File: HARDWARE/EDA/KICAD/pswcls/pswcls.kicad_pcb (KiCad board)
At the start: 2 copper layers, 60.9 x 27 mm, 22 parts, among them J1 PW_RELAY, J2 PW_LOGIC_RELAY, J3 RELAY_TERMINAL, J4 NC_Relay, J5 NA_Relay, J6 C_Relay, K1 G5LE-1, Q1 BC549, U1 4N35

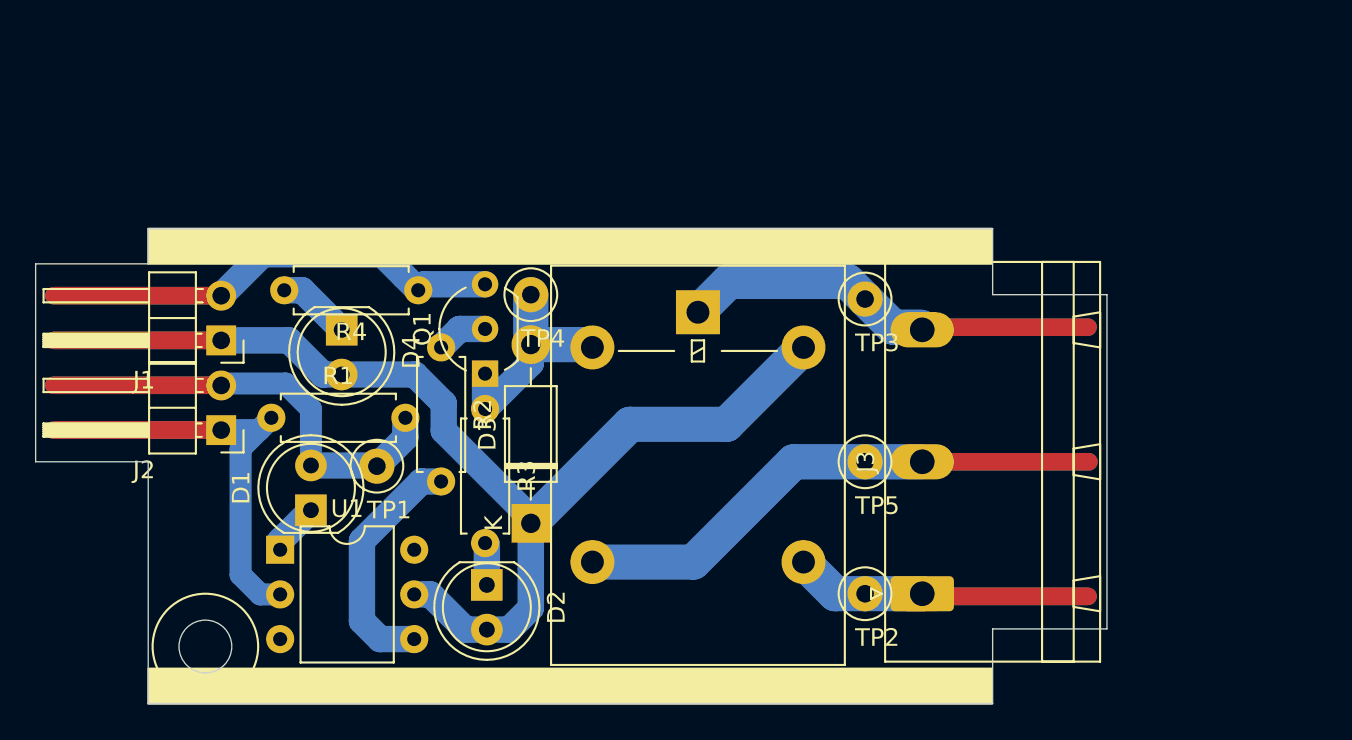
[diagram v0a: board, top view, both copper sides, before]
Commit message: pre adjust pcb and adjust schematic
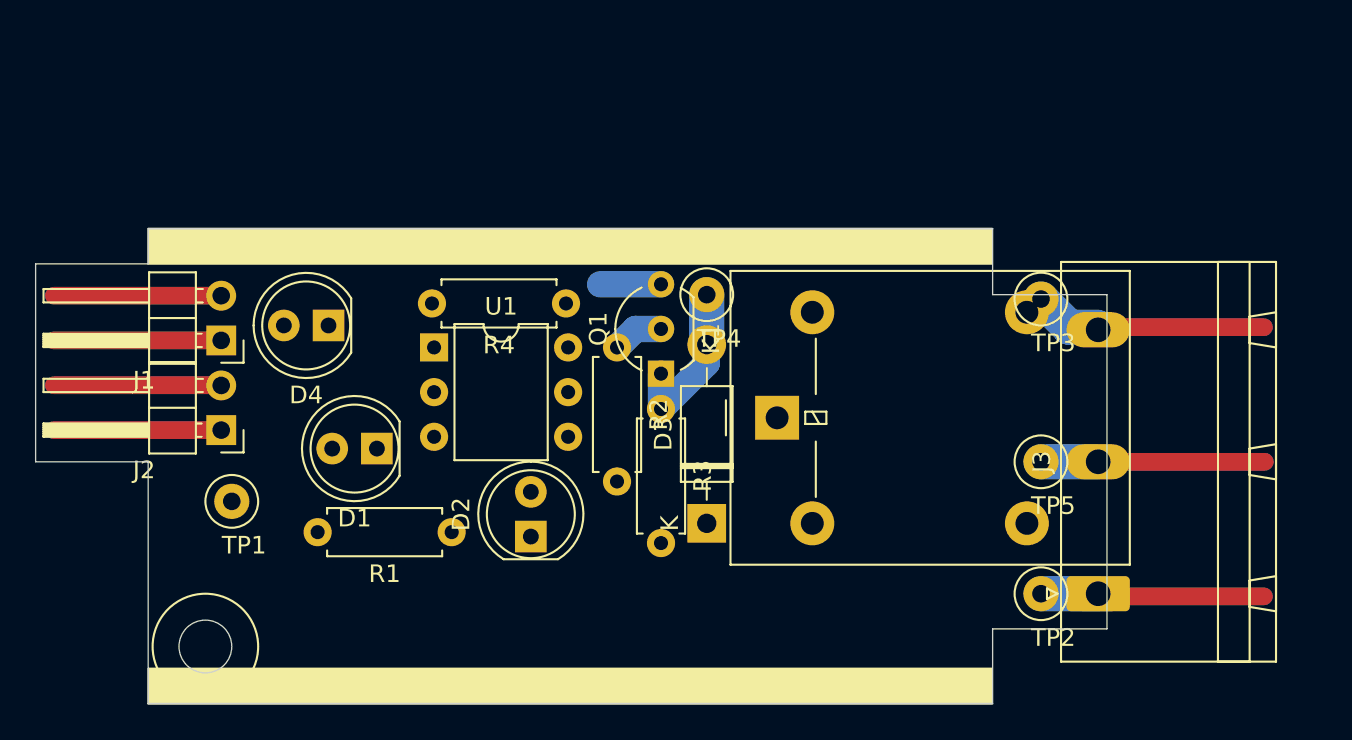
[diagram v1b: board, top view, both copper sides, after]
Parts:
- moved U1 14.5 mm to (128.0, 100.0)
- moved R1 12.1 mm to (129.0, 110.5), turned to 180 degrees
- moved D3 10.0 mm to (143.5, 110.0)
- moved J3 10.0 mm to (165.8, 114.0)
- moved J4 10.0 mm to (165.7, 114.2)
- moved J5 10.0 mm to (165.7, 106.5)
- moved J6 10.0 mm to (165.7, 98.8)
- moved Q1 10.0 mm to (140.9, 101.5)
- moved R2 10.0 mm to (138.4, 100.0)
- moved R3 10.0 mm to (140.9, 103.5)
- moved TP2 10.0 mm to (162.5, 114.0)
- moved TP3 10.0 mm to (162.5, 97.2)
- moved TP4 10.0 mm to (143.5, 97.0)
- moved TP5 10.0 mm to (162.5, 106.5)
- moved TP1 8.49 mm to (116.5, 108.8)
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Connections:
- K1 pad 2: Net-(D3-Pad2) -> vcc_relay
- K1 pad 5: vcc_relay -> Net-(D3-Pad2)
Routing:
- net vcc_relay: track 74.5 -> 19.0 mm
- net NA_Relay: track 40.2 -> 22.3 mm
- net vll_relay: track 35.2 -> 19.0 mm
- net GNDD: track 34.5 -> 19.0 mm
- net Net-(R2-Pad2): track 13.9 -> 0.00 mm
- net GNDA: track 36.0 -> 22.5 mm
- net C_Relay: track 33.5 -> 22.8 mm
- net NC_Relay: track 26.4 -> 22.2 mm
- net Net-(D4-Pad1): track 4.20 -> 0.00 mm
- net Net-(D3-Pad2): track 13.2 -> 9.59 mm
- net Net-(D1-Pad1): track 2.97 -> 0.00 mm
- net Net-(D2-Pad1): track 2.42 -> 0.00 mm

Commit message: finished remix
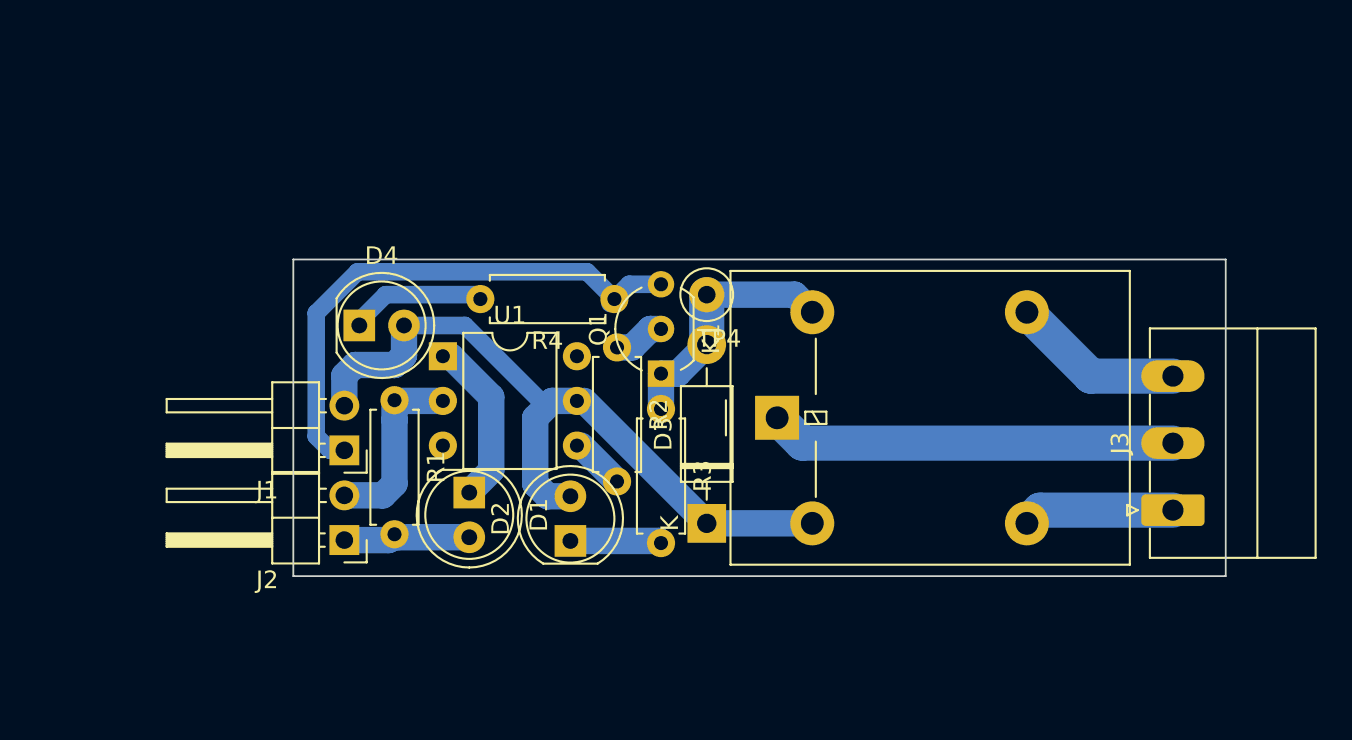
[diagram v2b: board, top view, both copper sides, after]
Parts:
- removed J4: NC_Relay, Connector_PinHeader_2.54mm:PinHeader_1x01_P2.54mm_Horizontal
- removed J5: NA_Relay, Connector_PinHeader_2.54mm:PinHeader_1x01_P2.54mm_Horizontal
- removed J6: C_Relay, Connector_PinHeader_2.54mm:PinHeader_1x01_P2.54mm_Horizontal
- removed TP1: Logic_Value, TestPoint:TestPoint_Loop_D1.80mm_Drill1.0mm_Beaded
- removed TP2: NC_Relay, TestPoint:TestPoint_Loop_D1.80mm_Drill1.0mm_Beaded
- removed TP3: C_Relay, TestPoint:TestPoint_Loop_D1.80mm_Drill1.0mm_Beaded
- removed TP5: NA_Relay, TestPoint:TestPoint_Loop_D1.80mm_Drill1.0mm_Beaded
- J3: footprint Connector_Phoenix_GMSTB:PhoenixContact_GMSTBA_2,5_3-G_1x03_P7.50mm_Horizontal -> Connector_Phoenix_MC:PhoenixContact_MC_1,5_3-G-3.81_1x03_P3.81mm_Horizontal
- moved J1 9.38 mm to (122.9, 105.8)
- moved J2 9.38 mm to (122.9, 111.0)
- moved R1 8.17 mm to (125.8, 103.0), turned to 270 degrees
- moved J3 6.37 mm to (170.0, 109.2)
- moved D1 5.81 mm to (130.0, 108.2), turned to 270 degrees
- moved R4 2.76 mm to (138.2, 97.2)
- moved D2 2.26 mm to (135.8, 111.0)
- moved D4 1.75 mm to (123.8, 98.8), turned to 0 degrees
- moved U1 0.71 mm to (128.5, 100.5)
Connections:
- J1 pad 1: vcc_relay -> GNDA
- J1 pad 2: GNDA -> vcc_relay
- J2 pad 1: GNDD -> vll_relay
- J2 pad 2: vll_relay -> GNDD
- J3 pad 1: NC_Relay -> NA_Relay
- J3 pad 2: NA_Relay -> C_Relay
- J3 pad 3: C_Relay -> NC_Relay
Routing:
- net vcc_relay: track 19.0 -> 44.2 mm
- net NA_Relay: track 22.3 -> 8.61 mm
- net NC_Relay: track 22.2 -> 9.80 mm
- net vll_relay: track 19.0 -> 7.31 mm
- net Net-(D1-Pad1): track 0.00 -> 9.66 mm
- net GNDD: track 19.0 -> 10.6 mm
- net GNDA: track 22.5 -> 30.8 mm
- net Net-(D4-Pad1): track 0.00 -> 7.85 mm
- net Net-(D2-Pad1): track 0.00 -> 5.20 mm
- net Net-(D3-Pad2): track 9.59 -> 14.5 mm
- net Net-(R2-Pad2): track 0.00 -> 2.88 mm
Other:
- board size 60.9 x 27 mm -> 53 x 18 mm
- net class Default: clearance 0.5 -> 0.25
- rule trace_clearance: 0.5 -> 0.25

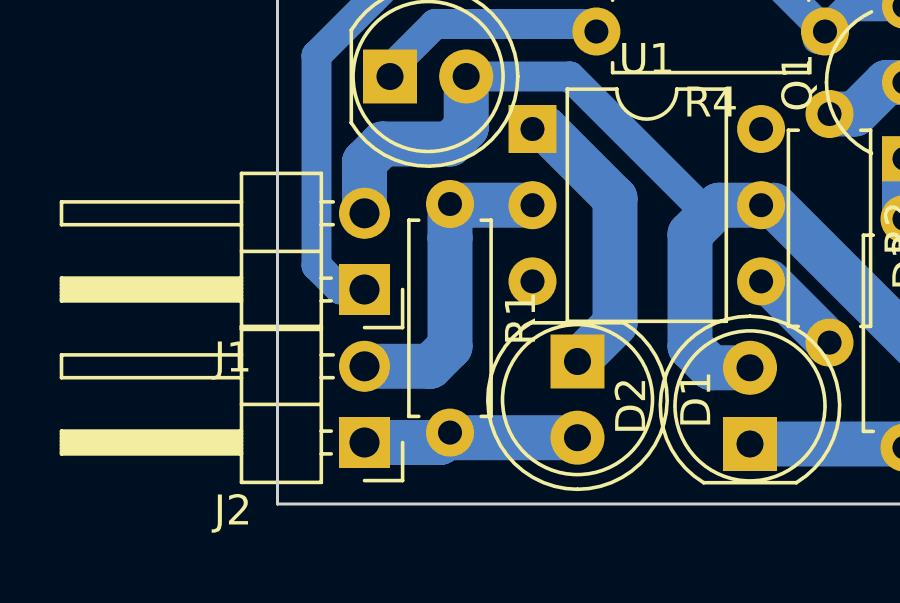
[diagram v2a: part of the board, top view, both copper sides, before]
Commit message: adjust project, problem report
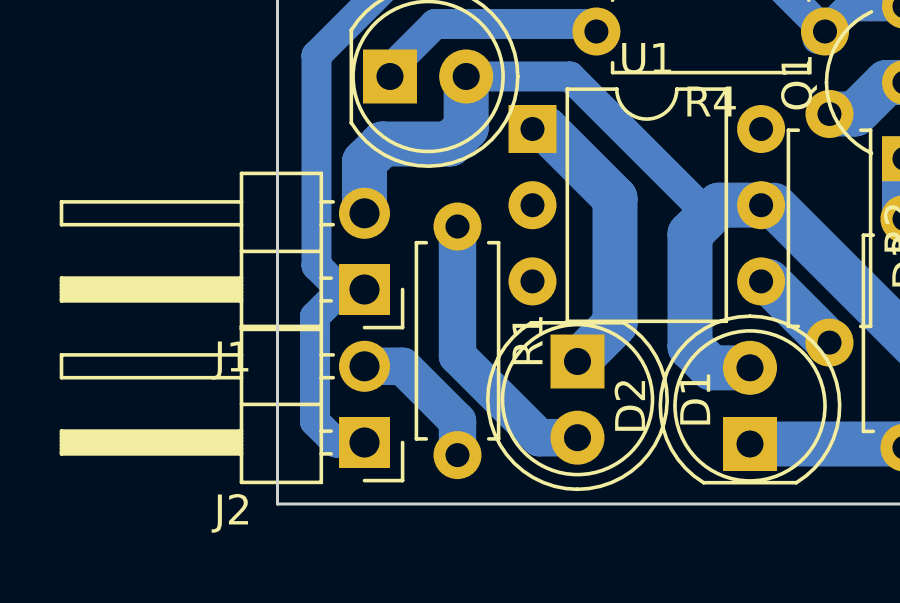
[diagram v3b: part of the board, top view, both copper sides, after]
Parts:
- R1: value 120K -> 330R
- R2: value 10K -> 12K
- R3: value 100R -> 330R
- R4: value 120R -> 330R
- moved R1 0.79 mm to (126.0, 103.8)
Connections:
- D1 pad 2: vll_relay -> Net-(D1-Pad2)
- J2 pad 1: vll_relay -> GNDA
- J2 pad 2: GNDD -> vll_relay
- R1 pad 1: GNDD -> Net-(D1-Pad2)
- U1 pad 2: GNDD -> GNDA
- U1 pad 3: Net-(U1-Pad3) -> (no net)
- U1 pad 6: Net-(U1-Pad6) -> (no net)
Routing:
- net GNDD: track 10.6 -> 0.00 mm
- net Net-(D1-Pad2): track 0.00 -> 9.50 mm
- net GNDA: track 30.8 -> 38.3 mm
- net vll_relay: track 7.31 -> 4.99 mm

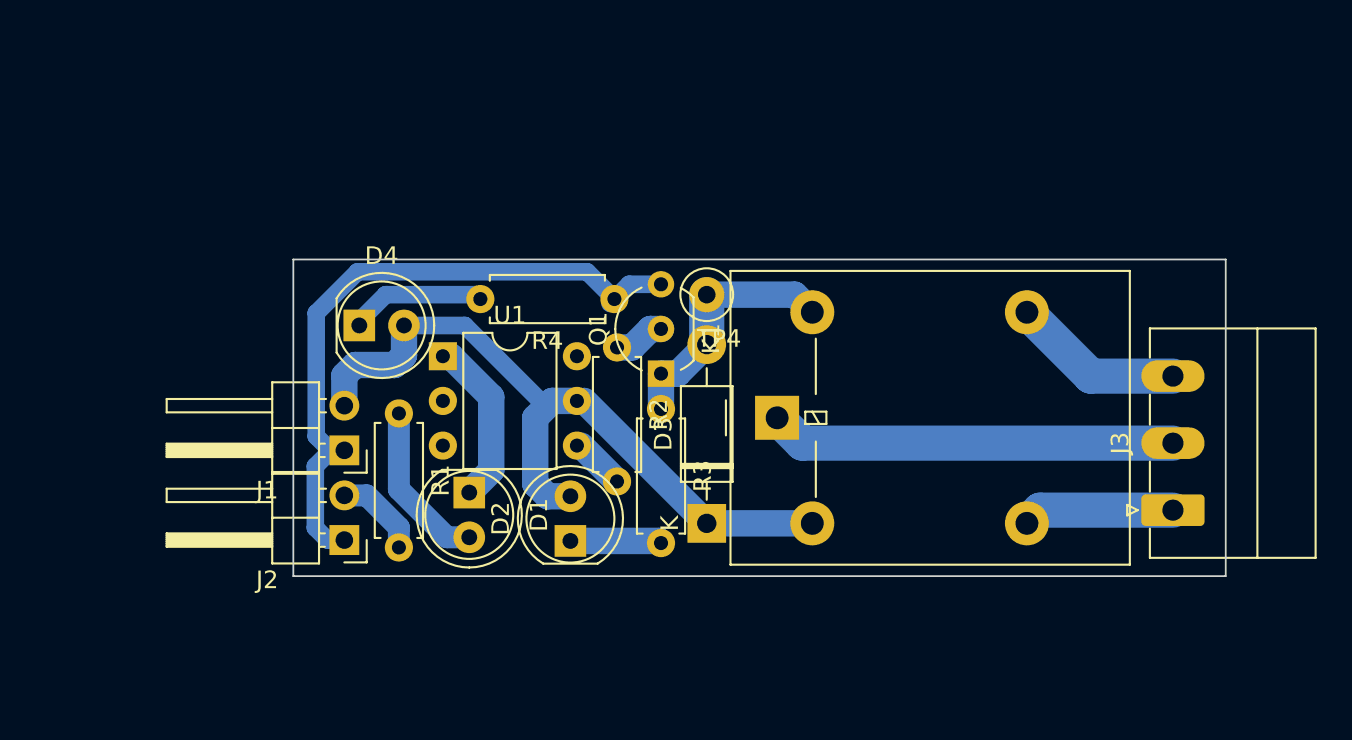
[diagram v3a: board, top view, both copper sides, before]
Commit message: adjust project, FINISHED
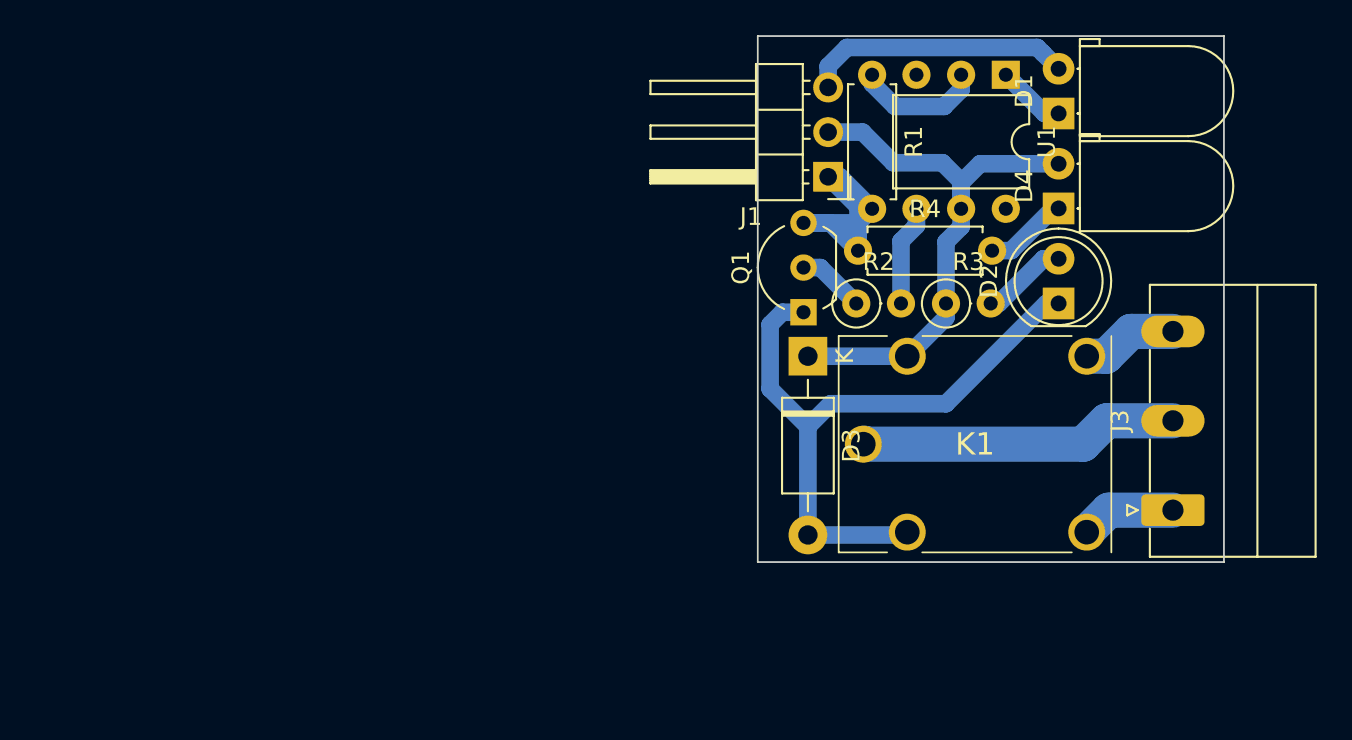
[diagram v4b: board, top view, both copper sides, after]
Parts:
- removed J2: PW_LOGIC_RELAY, Connector_PinHeader_2.54mm:PinHeader_1x02_P2.54mm_Horizontal
- removed TP4: !Power_Relay, TestPoint:TestPoint_Loop_D1.80mm_Drill1.0mm_Beaded
- D1: footprint LED_THT:LED_D5.0mm_Clear -> LED_THT:LED_D5.0mm_Horizontal_O1.27mm_Z3.0mm_Clear
- D4: footprint LED_THT:LED_D5.0mm -> LED_THT:LED_D5.0mm_Horizontal_O1.27mm_Z3.0mm
- J1: value PW_RELAY -> CONN; footprint Connector_PinHeader_2.54mm:PinHeader_1x02_P2.54mm_Horizontal -> Connector_PinHeader_2.54mm:PinHeader_1x03_P2.54mm_Horizontal
- J3: footprint Connector_Phoenix_MC:PhoenixContact_MC_1,5_3-G-3.81_1x03_P3.81mm_Horizontal -> Connector_Phoenix_MC_HighVoltage:PhoenixContact_MC_1,5_3-G-5.08_1x03_P5.08mm_Horizontal
- K1: value G5LE-1 -> SRA-12VDC-CL-REMIX; footprint RELAY_THT_PROJECT:RELAY_SPDT-G5LE-1-5V -> SRA-12VDC-CL:SRA12VDCCL
- R2, R3: footprint Resistor_THT:R_Axial_DIN0207_L6.3mm_D2.5mm_P7.62mm_Horizontal -> Resistor_THT:R_Axial_DIN0207_L6.3mm_D2.5mm_P2.54mm_Vertical
- moved D4 40.3 mm to (163.5, 92.1), turned to 90 degrees
- moved D1 39.8 mm to (163.5, 86.7), turned to 90 degrees
- moved U1 35.8 mm to (160.5, 84.5), turned to 270 degrees
- moved R1 33.1 mm to (152.9, 84.5)
- moved J1 31.6 mm to (150.4, 90.3)
- moved D2 30.9 mm to (163.5, 97.5)
- moved R3 17.3 mm to (157.1, 97.5), turned to 0 degrees
- moved R4 14.1 mm to (152.1, 94.5), turned to 0 degrees
- moved R2 13.8 mm to (152.0, 97.5), turned to 0 degrees
- moved K1 11.3 mm to (158.8, 105.5), turned to 0 degrees
- moved D3 11.1 mm to (149.2, 100.5), turned to 270 degrees
- moved Q1 8.82 mm to (149.0, 98.0)
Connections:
- D1 pad 2: Net-(D1-Pad2) -> vll_relay
- D2 pad 2: vcc_relay -> Net-(D2-Pad2)
- D3 pad 2: Net-(D3-Pad2) -> Net-(D2-Pad1)
- J3 pad 1: NA_Relay -> NC_Relay
- J3 pad 3: NC_Relay -> NA_Relay
- K1 pad 5: Net-(D3-Pad2) -> Net-(D2-Pad1)
- Q1 pad 1: Net-(D3-Pad2) -> Net-(D2-Pad1)
- R1 pad 1: Net-(D1-Pad2) -> Net-(R1-Pad1)
- R1 pad 2: vll_relay -> GNDA
- R3 pad 1: Net-(D3-Pad2) -> vcc_relay
- R3 pad 2: Net-(D2-Pad1) -> Net-(D2-Pad2)
- U1 pad 2: GNDA -> Net-(R1-Pad1)
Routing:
- net Net-(D2-Pad1): track 5.20 -> 37.9 mm
- net GNDA: track 38.3 -> 17.7 mm
- net Net-(D3-Pad2): track 14.5 -> 0.00 mm
- net vcc_relay: track 44.2 -> 33.9 mm
- net vll_relay: track 4.99 -> 15.2 mm
- net Net-(D1-Pad2): track 9.50 -> 0.00 mm
- net Net-(R1-Pad1): track 0.00 -> 7.34 mm
- net Net-(D1-Pad1): track 9.66 -> 3.91 mm
- net Net-(D2-Pad2): track 0.00 -> 4.91 mm
- net C_Relay: track 23.1 -> 18.2 mm
- net NC_Relay: track 9.80 -> 5.42 mm
- net NA_Relay: track 8.61 -> 5.48 mm
- net Net-(R2-Pad2): track 2.88 -> 5.74 mm
- net Net-(D4-Pad1): track 7.85 -> 5.27 mm
- net Net-(Q1-Pad2): track 2.93 -> 3.84 mm
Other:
- board size 53 x 18 mm -> 26.5 x 29.9 mm
